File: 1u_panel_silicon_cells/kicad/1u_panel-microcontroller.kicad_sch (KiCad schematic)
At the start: 43 parts, among them J2 2-1734592-0, U1 TCAN330GDCNT, U11 TMP101NA/3KSLOTTED, U2 TMP101NA/3KSLOTTED, U7 STM32F091CCT7, X1 ECS-160-10-36Q-ES-TR

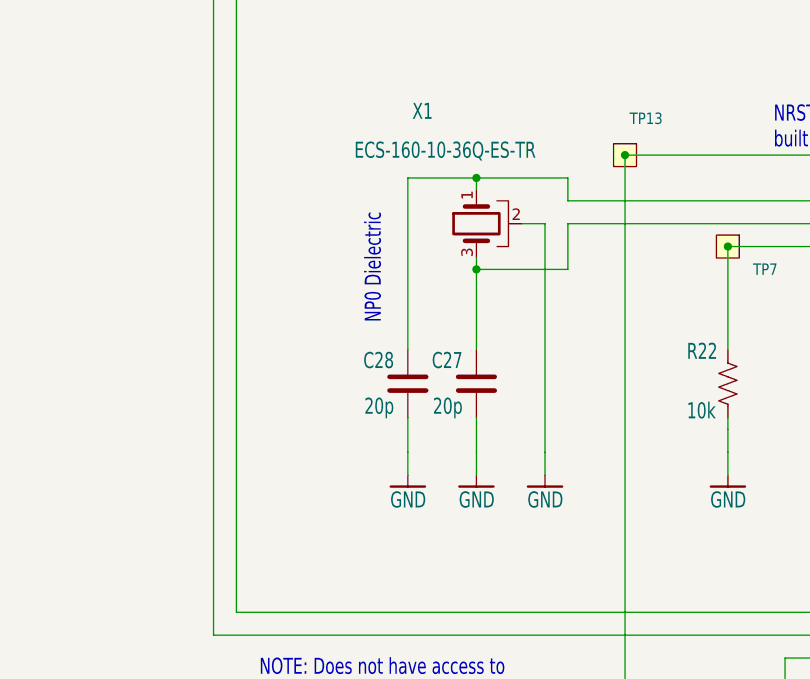
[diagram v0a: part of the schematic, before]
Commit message: final changes for silicon solar module
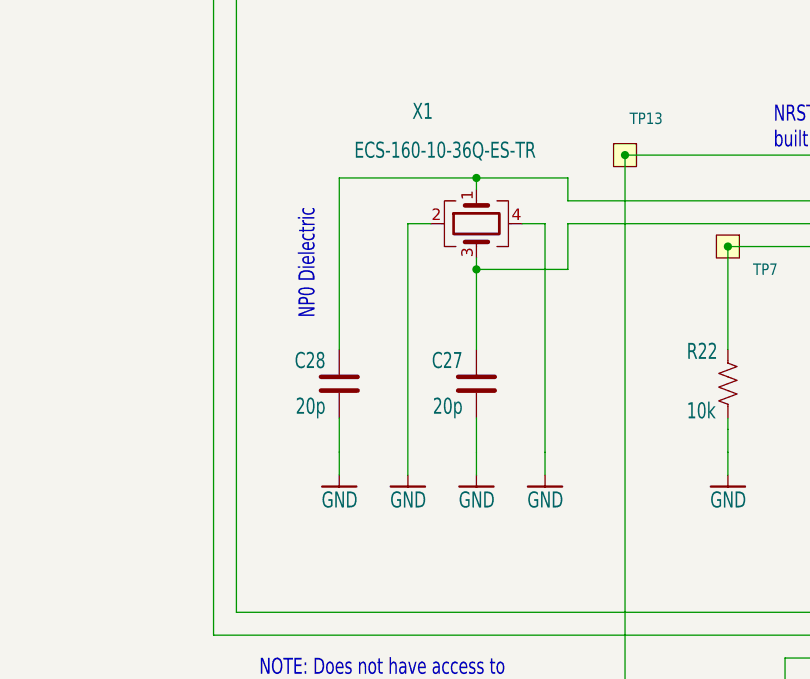
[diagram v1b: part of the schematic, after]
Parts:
- X1: footprint Crystal:Crystal_SMD_2520-4Pin_2.5x2.0mm -> oresat-misc:ECS-160-10-36Q-ES-TR; symbol Device:Crystal_GND2 -> Device:Crystal_GND24
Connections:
- net GND: now also X1.4
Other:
- moved on the sheet: C28
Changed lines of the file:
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@@
 	(wire
 		(pts
-			(xy 166.37 115.57) (xy 166.37 96.52)
+			(xy 158.75 115.57) (xy 158.75 96.52)
 		)
 		(stroke
@@
 	(wire
 		(pts
-			(xy 166.37 127) (xy 166.37 129.54)
+			(xy 158.75 127) (xy 158.75 129.54)
 		)
 		(stroke
@@
 	(wire
 		(pts
+			(xy 166.37 101.6) (xy 166.37 129.54)
+		)
+		(stroke
+			(width 0)
+			(type default)
+		)
+	)
+	(wire
+		(pts
 			(xy 250.19 73.66) (xy 250.19 76.2)
 		)
@@
 	(wire
 		(pts
+			(xy 168.91 101.6) (xy 166.37 101.6)
+		)
+		(stroke
+			(width 0)
+			(type default)
+		)
+	)
+	(wire
+		(pts
 			(xy 299.72 184.15) (xy 110.49 184.15)
 		)
@@
 	(wire
 		(pts
-			(xy 166.37 96.52) (xy 173.99 96.52)
+			(xy 158.75 96.52) (xy 173.99 96.52)
 		)
 		(stroke
@@
 	(wire
 		(pts
-			(xy 166.37 127) (xy 166.37 123.19)
+			(xy 158.75 127) (xy 158.75 123.19)
 		)
 		(stroke
@@
 	(text "NP0 Dielectric"
 		(exclude_from_sim no)
-		(at 163.576 112.776 90)
+		(at 156.21 112.268 90)
 		(effects
 			(font
@@
 	(symbol
 		(lib_id "oresat-power:GND")
+		(at 166.37 129.54 0)
+		(mirror y)
+		(unit 1)
+		(exclude_from_sim no)
+		(in_bom yes)
+		(on_board yes)
+		(dnp no)
+		(property "Reference" "#GND010"
+			(at 166.37 129.54 0)
+			(effects
+				(font
+					(size 1.27 1.27)
+				)
+				(hide yes)
+			)
+		)
+		(property "Value" "GND"
+			(at 168.402 133.35 0)
+			(effects
+				(font
+					(size 1.778 1.27)
+				)
+				(justify left bottom)
+			)
+		)
+		(property "Footprint" ""
+			(at 166.37 130.81 0)
+			(effects
+				(font
+					(size 1.27 1.27)
+				)
+				(hide yes)
+			)
+		)
+		(property "Datasheet" ""
+			(at 166.37 130.81 0)
+			(effects
+				(font
+					(size 1.27 1.27)
+				)
+				(hide yes)
+			)
+		)
+		(property "Description" "Power symbol creates a global label with name \"GND\" , ground"
+			(at 166.37 129.54 0)
+			(effects
+				(font
+					(size 1.27 1.27)
+				)
+				(hide yes)
+			)
+		)
+		(pin "1"
+		)
+		(instances
+			(project "1u_panel-silicon"
+				(path "/115bd2cd-7c08-4b54-867b-a326ee0699c1/bfa81e66-0bc2-4d21-a09c-e64719ae80bc"
+					(reference "#GND010")
+					(unit 1)
+				)
+			)
+		)
+	)
+	(symbol
+		(lib_id "oresat-power:GND")
 		(at 215.9 233.68 0)
 		(mirror y)
@@
 	)
 	(symbol
-		(lib_id "Device:Crystal_GND2")
+		(lib_id "Device:Crystal_GND24")
 		(at 173.99 101.6 90)
 		(mirror x)
@@
 			)
 		)
-		(property "Footprint" "Crystal:Crystal_SMD_2520-4Pin_2.5x2.0mm"
+		(property "Footprint" "oresat-misc:ECS-160-10-36Q-ES-TR"
 			(at 173.99 101.6 0)
 			(effects
@@
 			)
 		)
-		(property "Description" "Three pin crystal, GND on pin 2"
+		(property "Description" "Four pin crystal, GND on pins 2 and 4"
 			(at 173.99 101.6 0)
 			(effects
@@
 		(pin "3"
 		)
+		(pin "4"
+		)
 		(instances
 			(project "1u_panel-silicon"
@@
 	(symbol
 		(lib_id "Device:C")
-		(at 166.37 119.38 0)
+		(at 158.75 119.38 0)
 		(mirror y)
 		(unit 1)
@@
 		(dnp no)
 		(property "Reference" "C28"
-			(at 164.846 117.856 0)
+			(at 157.226 117.856 0)
 			(effects
 				(font
@@
 		)
 		(property "Value" "20p"
-			(at 164.846 122.936 0)
+			(at 157.226 122.936 0)
 			(effects
 				(font
@@
 		)
 		(property "Footprint" "oresat-passives:0603-C-NOSILK"
-			(at 165.4048 123.19 0)
+			(at 157.7848 123.19 0)
 			(effects
 				(font
@@
 		)
 		(property "Datasheet" "~"
-			(at 166.37 119.38 0)
+			(at 158.75 119.38 0)
 			(effects
 				(font
@@
 		)
 		(property "Description" "Unpolarized capacitor"
-			(at 166.37 119.38 0)
+			(at 158.75 119.38 0)
 			(effects
 				(font
@@
 		)
 		(property "DIS" "Digi-Key"
-			(at 166.37 119.38 0)
+			(at 158.75 119.38 0)
 			(effects
 				(font
@@
 		)
 		(property "DPN" "490-1334-2-ND"
-			(at 166.37 119.38 0)
+			(at 158.75 119.38 0)
 			(effects
 				(font
@@
 		)
 		(property "MFR" "Murata"
-			(at 166.37 119.38 0)
+			(at 158.75 119.38 0)
 			(effects
 				(font
@@
 		)
 		(property "MPN" "GRM1885C2A200JA01D"
-			(at 166.37 119.38 0)
+			(at 158.75 119.38 0)
 			(effects
 				(font
@@
 		)
 		(instances
-			(project "1u_panel-silicon"
+			(project ""
+				(path "/115bd2cd-7c08-4b54-867b-a326ee0699c1/5c4415f1-d90e-44ce-bb2c-b4c8edead48f"
+					(reference "C9")
+					(unit 1)
+				)
 				(path "/115bd2cd-7c08-4b54-867b-a326ee0699c1/bfa81e66-0bc2-4d21-a09c-e64719ae80bc"
 					(reference "C9")
@@
 	(symbol
 		(lib_id "oresat-power:GND")
-		(at 166.37 129.54 0)
+		(at 158.75 129.54 0)
 		(mirror y)
 		(unit 1)
@@
 		(dnp no)
 		(property "Reference" "#GND054"
-			(at 166.37 129.54 0)
+			(at 158.75 129.54 0)
 			(effects
 				(font
@@
 		)
 		(property "Value" "GND"
-			(at 168.402 133.35 0)
+			(at 160.782 133.35 0)
 			(effects
 				(font
@@
 		)
 		(property "Footprint" ""
-			(at 166.37 130.81 0)
+			(at 158.75 130.81 0)
 			(effects
 				(font
@@
 		)
 		(property "Datasheet" ""
-			(at 166.37 130.81 0)
+			(at 158.75 130.81 0)
 			(effects
 				(font
@@
 		)
 		(property "Description" "Power symbol creates a global label with name \"GND\" , ground"
-			(at 166.37 129.54 0)
+			(at 158.75 129.54 0)
 			(effects
 				(font
